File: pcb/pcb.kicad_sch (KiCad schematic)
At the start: 12 parts, among them CN1 1x3, CN2 1x8, CN3 1x8, CN4 1x8, CN5 1x4, CN6 1x2, CN7 1x2, SW1 switch_3x4, SW2 switch_3x4

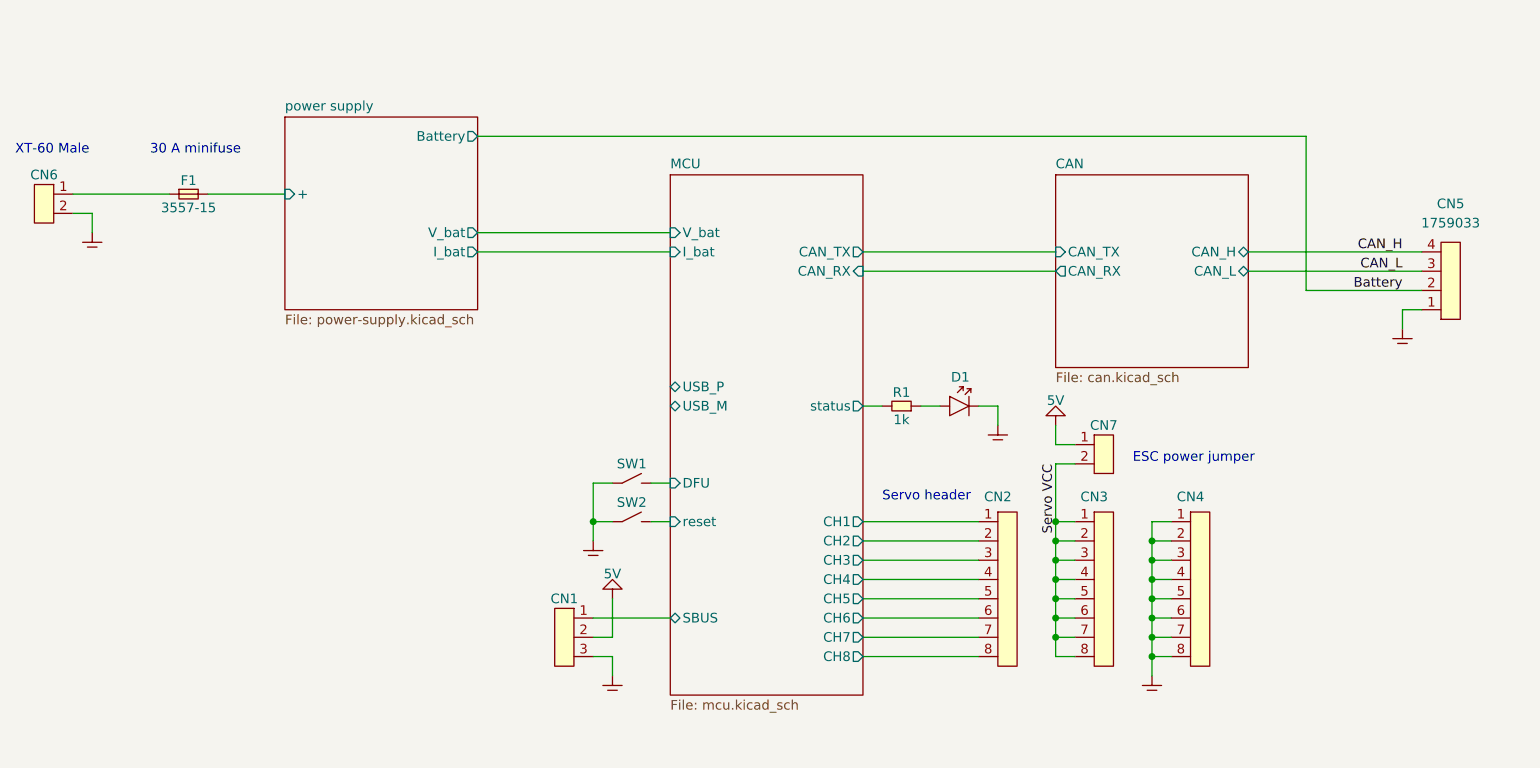
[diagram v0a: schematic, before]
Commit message: schematic mostly done
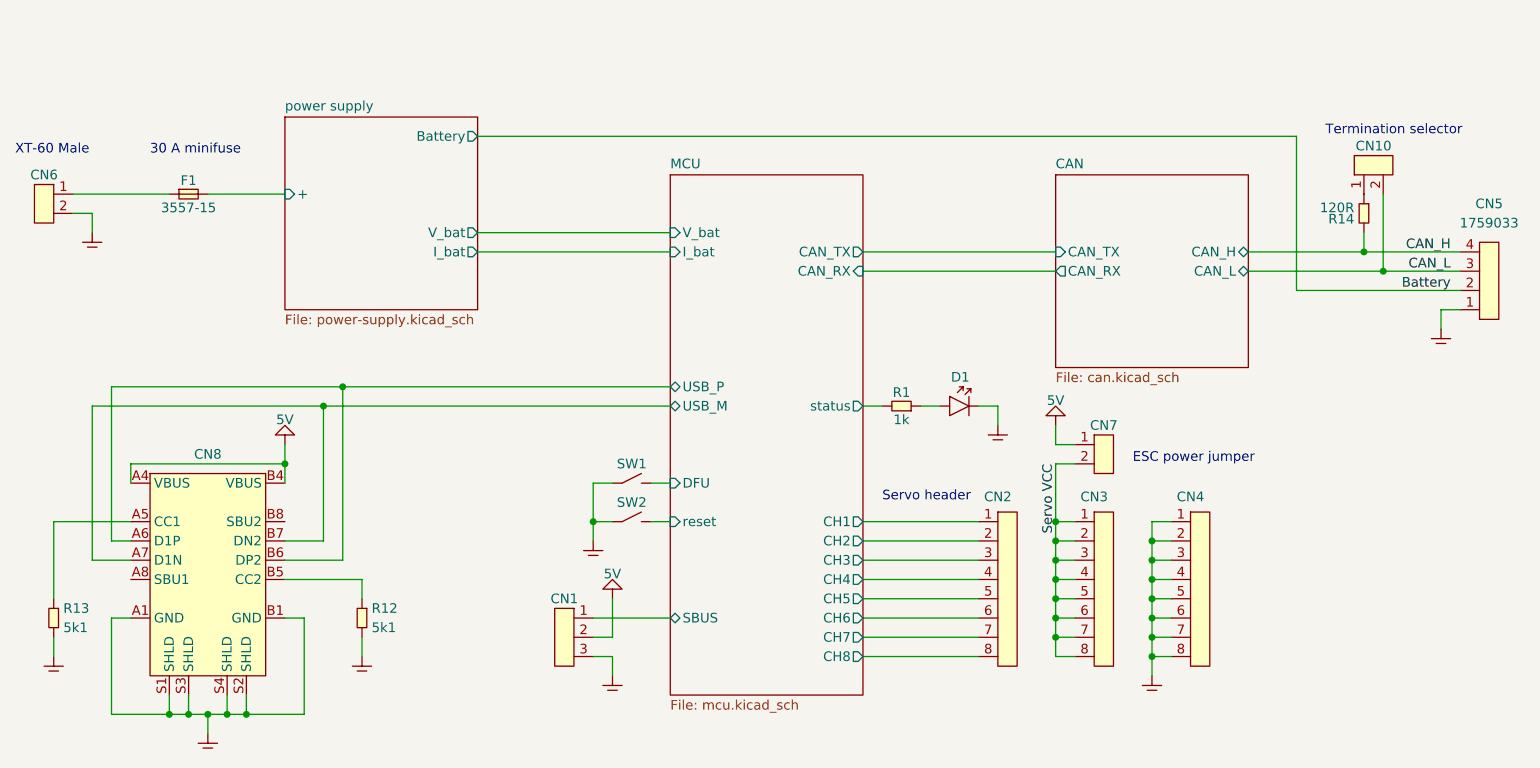
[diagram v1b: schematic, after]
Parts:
- added CN10: 1x2, symbol pin_headers:1x2
- added CN8: ~, USB:USB4105-GF-A, symbol connectors:USB4105-GF-A
- added R12, R13: 5k1, SMT:0603, symbol generic:R
- added R14: 120R, SMT:0603, symbol generic:R
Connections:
- net CAN_H: now also R14.2
- net CAN_L: now also CN10.2
- net GND: now also CN8.A1 (GND), CN8.A4 (VBUS), CN8.B1 (GND), CN8.B4 (VBUS), CN8.S1 (SHLD), CN8.S2 (SHLD), CN8.S3 (SHLD), CN8.S4 (SHLD), R12.2, R13.2
- net MCU/USB_M: now also CN8.A7 (D1N), CN8.B7 (DN2)
- net MCU/USB_P: now also CN8.A6 (D1P), CN8.B6 (DP2)
- new net: CN10.1, R14.1
- new net: CN8.A5 (CC1), R13.1
- new net: CN8.B5 (CC2), R12.1
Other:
- note added: "Termination selector"
- title: (none) -> CAN bus to RC servo adapter
- moved on the sheet: CN5

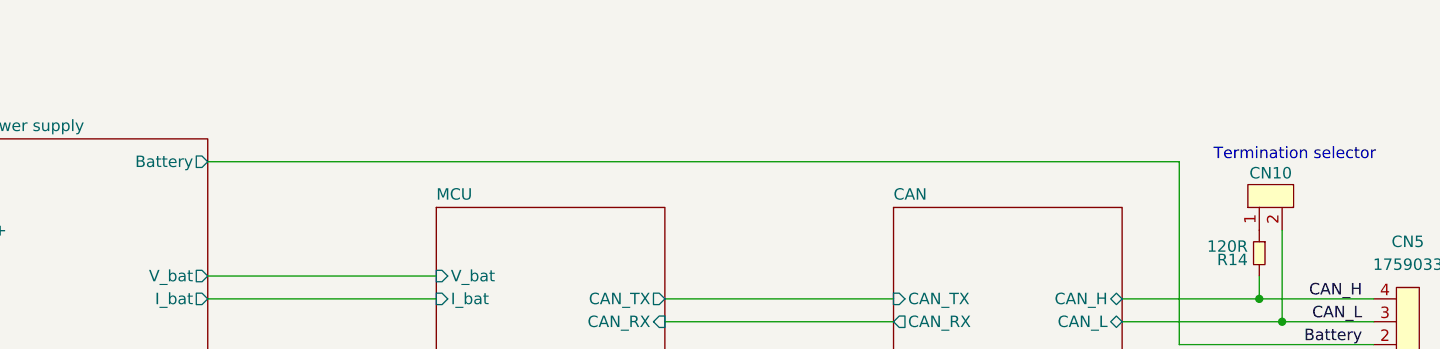
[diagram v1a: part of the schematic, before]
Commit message: started work on layout
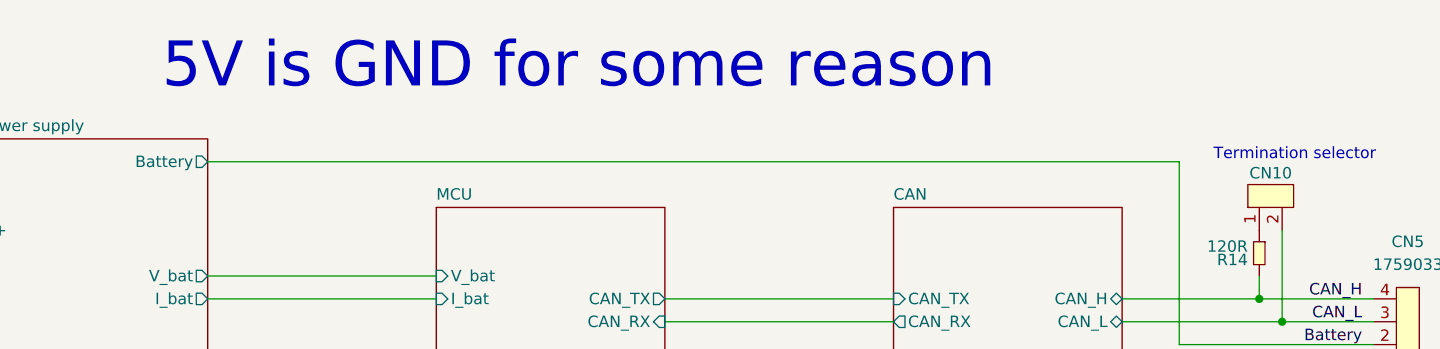
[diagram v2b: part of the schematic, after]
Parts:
- CN10, CN7: footprint (none) -> pin_headers:1x2
- CN2, CN3, CN4: footprint (none) -> pin_headers:1x8
- F1: footprint SMT:0603 -> (none)
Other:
- note added: "5V is GND for some reason"
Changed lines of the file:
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@@
   (title_block
     (title "CAN bus to RC servo adapter")
-    (date "2024-01-10")
+    (date "2024-01-14")
     (rev "0")
     (comment 1 "User interfaces")
@@
     (effects (font (size 1.27 1.27)) (justify left bottom))
   )
+  (text "5V is GND for some reason" (at 109.22 63.5 0)
+    (effects (font (size 5 5)) (justify left bottom))
+  )
   (text "ESC power jumper" (at 200.66 114.3 0)
     (effects (font (size 1.27 1.27)) (justify left bottom))
@@
   (symbol (lib_id "generic:5V") (at 88.9 111.76 0) (unit 1)
     (in_bom yes) (on_board yes) (dnp no)
-    (property "Reference" "5V04" (at 92.71 110.49 0)
+    (property "Reference" "#5V04" (at 92.71 110.49 0)
       (effects (font (size 1.27 1.27)) hide)
     )
@@
       (project "pcb"
         (path "/6bb3bad6-1a89-4624-b34d-6ddda7dd16d2"
-          (reference "5V04") (unit 1)
+          (reference "#5V04") (unit 1)
         )
       )
@@
       (effects (font (size 1.27 1.27)) hide)
     )
-    (property "Footprint" "" (at 231.14 78.74 0)
+    (property "Footprint" "pin_headers:1x2" (at 231.14 78.74 0)
       (effects (font (size 1.27 1.27)) hide)
     )
@@
   (symbol (lib_id "generic:GND") (at 132.08 142.24 0) (unit 1)
     (in_bom yes) (on_board yes) (dnp no) (fields_autoplaced)
-    (property "Reference" "GND07" (at 135.89 140.97 0)
+    (property "Reference" "#GND07" (at 135.89 140.97 0)
       (effects (font (size 1.27 1.27)) hide)
     )
@@
       (project "pcb"
         (path "/6bb3bad6-1a89-4624-b34d-6ddda7dd16d2"
-          (reference "GND07") (unit 1)
+          (reference "#GND07") (unit 1)
         )
       )
@@
       (effects (font (size 1.27 1.27)) hide)
     )
-    (property "Footprint" "" (at 193.04 121.92 0)
+    (property "Footprint" "pin_headers:1x8" (at 193.04 121.92 0)
       (effects (font (size 1.27 1.27)) hide)
     )
@@
   (symbol (lib_id "generic:GND") (at 129.54 124.46 0) (unit 1)
     (in_bom yes) (on_board yes) (dnp no) (fields_autoplaced)
-    (property "Reference" "GND01" (at 133.35 123.19 0)
+    (property "Reference" "#GND01" (at 133.35 123.19 0)
       (effects (font (size 1.27 1.27)) hide)
     )
@@
       (project "pcb"
         (path "/6bb3bad6-1a89-4624-b34d-6ddda7dd16d2"
-          (reference "GND01") (unit 1)
+          (reference "#GND01") (unit 1)
         )
       )
@@
   (symbol (lib_id "generic:GND") (at 203.2 142.24 0) (unit 1)
     (in_bom yes) (on_board yes) (dnp no) (fields_autoplaced)
-    (property "Reference" "GND09" (at 207.01 140.97 0)
+    (property "Reference" "#GND09" (at 207.01 140.97 0)
       (effects (font (size 1.27 1.27)) hide)
     )
@@
       (project "pcb"
         (path "/6bb3bad6-1a89-4624-b34d-6ddda7dd16d2"
-          (reference "GND09") (unit 1)
+          (reference "#GND09") (unit 1)
         )
       )
@@
       (effects (font (size 1.27 1.27)) hide)
     )
-    (property "Footprint" "" (at 205.74 121.92 0)
+    (property "Footprint" "pin_headers:1x8" (at 205.74 121.92 0)
       (effects (font (size 1.27 1.27)) hide)
     )
@@
       (effects (font (size 1.27 1.27)) hide)
     )
-    (property "Footprint" "" (at 180.34 121.92 0)
+    (property "Footprint" "pin_headers:1x8" (at 180.34 121.92 0)
       (effects (font (size 1.27 1.27)) hide)
     )
@@
         )
         (path "/6bb3bad6-1a89-4624-b34d-6ddda7dd16d2"
-          (reference "GND08") (unit 1)
+          (reference "#GND08") (unit 1)
         )
       )
@@
   (symbol (lib_id "generic:GND") (at 182.88 109.22 0) (unit 1)
     (in_bom yes) (on_board yes) (dnp no) (fields_autoplaced)
-    (property "Reference" "GND010" (at 186.69 107.95 0)
+    (property "Reference" "#GND010" (at 186.69 107.95 0)
       (effects (font (size 1.27 1.27)) hide)
     )
@@
       (project "pcb"
         (path "/6bb3bad6-1a89-4624-b34d-6ddda7dd16d2"
-          (reference "GND010") (unit 1)
+          (reference "#GND010") (unit 1)
         )
       )
@@
       (effects (font (size 1.27 1.27)) hide)
     )
-    (property "Footprint" "SMT:0603" (at 73.66 79.375 0)
+    (property "Footprint" "" (at 73.66 79.375 0)
       (effects (font (size 1.27 1.27)) hide)
     )
@@
   (symbol (lib_name "GND_1") (lib_id "generic:GND") (at 78.74 149.86 0) (unit 1)
     (in_bom yes) (on_board yes) (dnp no) (fields_autoplaced)
-    (property "Reference" "#GND01" (at 82.55 148.59 0)
+    (property "Reference" "#GND034" (at 82.55 148.59 0)
       (effects (font (size 1.27 1.27)) hide)
     )
@@
       (project "pcb"
         (path "/6bb3bad6-1a89-4624-b34d-6ddda7dd16d2"
-          (reference "#GND01") (unit 1)
+          (reference "#GND034") (unit 1)
         )
       )
@@
   (symbol (lib_id "generic:5V") (at 190.5 109.22 0) (unit 1)
     (in_bom yes) (on_board yes) (dnp no)
-    (property "Reference" "5V03" (at 194.31 107.95 0)
+    (property "Reference" "#5V03" (at 194.31 107.95 0)
       (effects (font (size 1.27 1.27)) hide)
     )
@@
       (project "pcb"
         (path "/6bb3bad6-1a89-4624-b34d-6ddda7dd16d2"
-          (reference "5V03") (unit 1)
+          (reference "#5V03") (unit 1)
         )
       )
@@
   (symbol (lib_id "generic:GND") (at 63.5 83.82 0) (unit 1)
     (in_bom yes) (on_board yes) (dnp no) (fields_autoplaced)
-    (property "Reference" "GND016" (at 67.31 82.55 0)
+    (property "Reference" "#GND016" (at 67.31 82.55 0)
       (effects (font (size 1.27 1.27)) hide)
     )
@@
       (project "pcb"
         (path "/6bb3bad6-1a89-4624-b34d-6ddda7dd16d2"
-          (reference "GND016") (unit 1)
+          (reference "#GND016") (unit 1)
         )
       )
@@
       (effects (font (size 1.27 1.27)) hide)
     )
-    (property "Footprint" "" (at 193.04 111.76 0)
+    (property "Footprint" "pin_headers:1x2" (at 193.04 111.76 0)
       (effects (font (size 1.27 1.27)) hide)
     )
@@
   (symbol (lib_id "generic:5V") (at 132.08 132.08 0) (unit 1)
     (in_bom yes) (on_board yes) (dnp no)
-    (property "Reference" "5V02" (at 135.89 130.81 0)
+    (property "Reference" "#5V02" (at 135.89 130.81 0)
       (effects (font (size 1.27 1.27)) hide)
     )
@@
       (project "pcb"
         (path "/6bb3bad6-1a89-4624-b34d-6ddda7dd16d2"
-          (reference "5V02") (unit 1)
-        )
-      )
+          (reference "#5V02") (unit 1)
+        )
+      )
